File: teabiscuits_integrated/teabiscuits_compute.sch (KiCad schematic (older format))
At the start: 38 parts, among them J1 Barrel_Jack, J10 Conn_Coaxial, J2 Conn_02x04_Odd_Even, J3 Conn_01x03, J4 Conn_01x03, J5 Conn_02x03_Odd_Even, J6 J1B1211CCD, J7 Conn_Coaxial, J8 Conn_Coaxial, J9 Conn_01x03, U1 teensy41, U2 OP07, U3 OP07, U4 TLE2426xP, U5 LF398_SOIC8, U7 REF5025AD

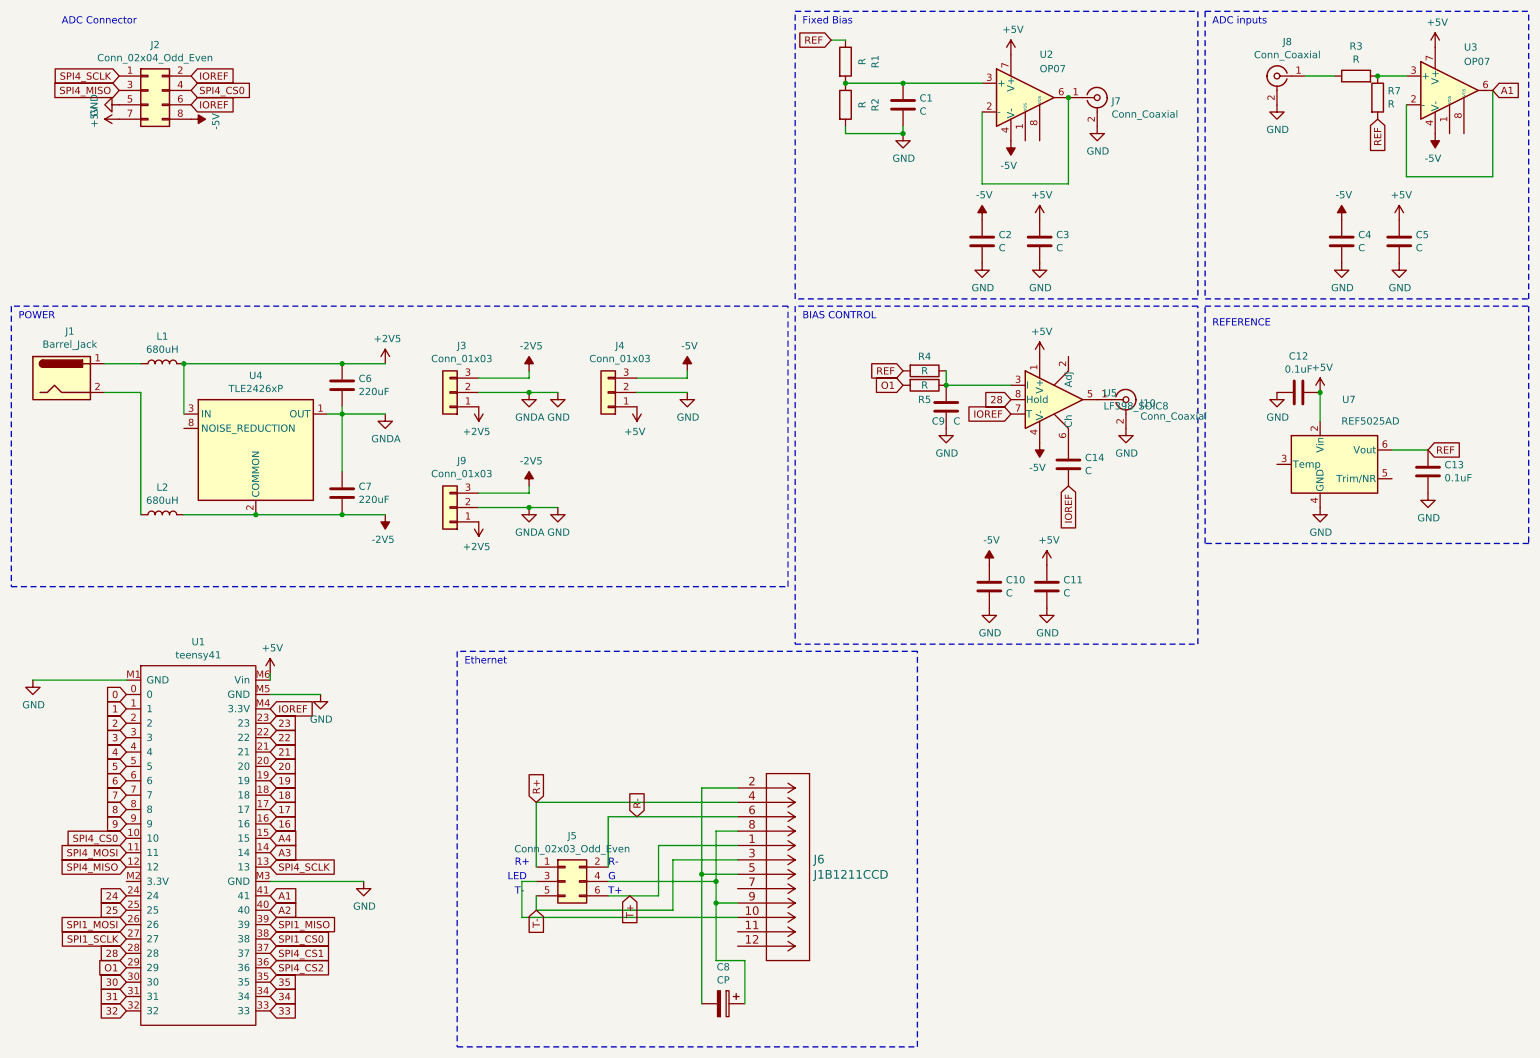
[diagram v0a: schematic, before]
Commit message: r4 of integrated pcb
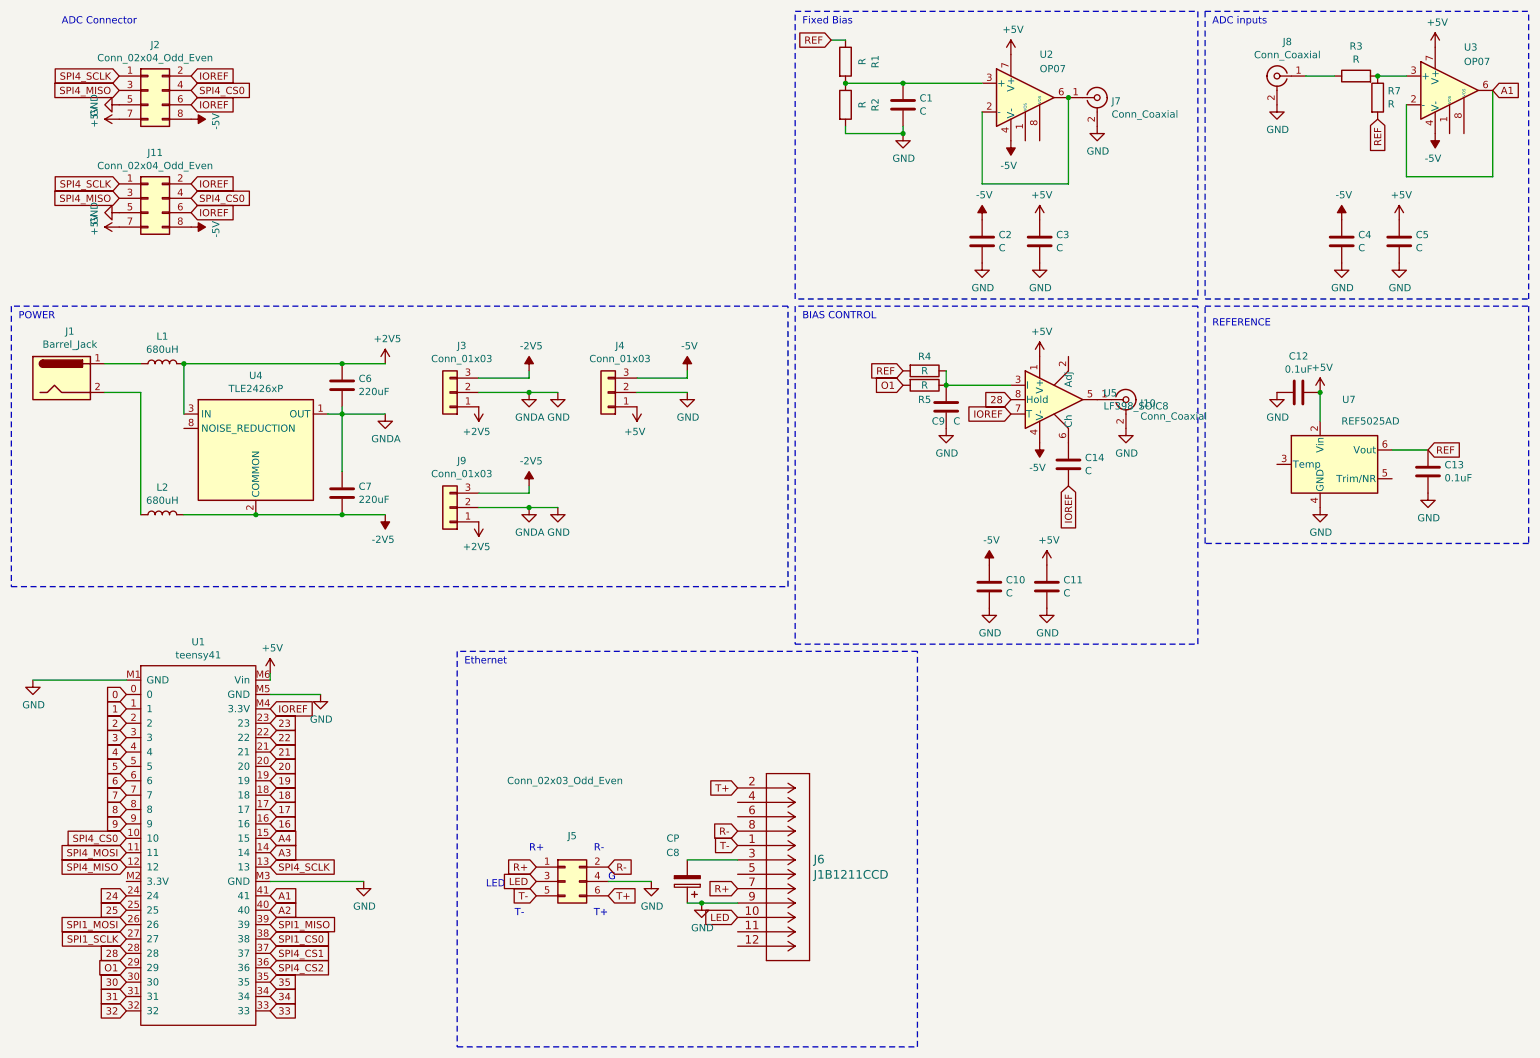
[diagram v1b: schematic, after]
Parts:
- added J11: Conn_02x04_Odd_Even, Connector_PinHeader_2.54mm:PinHeader_2x04_P2.54mm_Vertical, symbol Connector_Generic:Conn_02x04_Odd_Even
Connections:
- net +5V: now also J11.7 (Pin_7)
- net -5V: now also J11.8 (Pin_8)
- net GND: now also C8.1, J5.4 (Pin_4), J6.9, J11.5 (Pin_5)
- net IOREF: now also J11.2 (Pin_2), J11.6 (Pin_6)
- net R+: now also J6.7; no longer J6.4
- net R-: now also J6.8; no longer J6.6
- net SPI4_CS0: now also J11.4 (Pin_4)
- net SPI4_MISO: now also J11.3 (Pin_3)
- net SPI4_SCLK: now also J11.1 (Pin_1)
- net T+: now also J6.2; no longer J6.1
- net T-: now also J6.1; no longer J6.3
- net LED: now reaches J5.3 (Pin_3), J6.10
- new net: C8.2, J6.3
- now unconnected: J6.5
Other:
- moved on the sheet: C8
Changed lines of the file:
@@
 P 4450 6550
 F 0 "J5" H 4500 6867 50  0000 C CNN
-F 1 "Conn_02x03_Odd_Even" H 4500 6776 50  0000 C CNN
+F 1 "Conn_02x03_Odd_Even" H 4450 7250 50  0000 C CNN
 F 2 "Connector_PinHeader_2.00mm:PinHeader_2x03_P2.00mm_Vertical" H 4450 6550 50  0001 C CNN
 F 3 "~" H 4450 6550 50  0001 C CNN
@@
 L Device:CP C8
 U 1 1 5F594A00
-P 5550 7400
-F 0 "C8" V 5295 7400 50  0000 C CNN
-F 1 "CP" V 5386 7400 50  0000 C CNN
-F 2 "Capacitor_THT:C_Rect_L4.0mm_W2.5mm_P2.50mm" H 5588 7250 50  0001 C CNN
-F 3 "~" H 5550 7400 50  0001 C CNN
-	1    5550 7400
-	0    1    1    0
+P 5300 6550
+F 0 "C8" H 5400 6350 50  0000 C CNN
+F 1 "CP" H 5400 6250 50  0000 C CNN
+F 2 "Capacitor_THT:C_Rect_L4.0mm_W2.5mm_P2.50mm" H 5338 6400 50  0001 C CNN
+F 3 "~" H 5300 6550 50  0001 C CNN
+	1    5300 6550
+	-1   0    0    1
 $EndComp
 Wire Notes Line
@@
 	4400 3950 4200 3950
 Connection ~ 4200 3950
-Text Notes 4100 6450 0    50   ~ 0
+Text Notes 4200 6350 0    50   ~ 0
 R+
-Text Notes 4750 6450 0    50   ~ 0
+Text Notes 4650 6350 0    50   ~ 0
 R-
-Text Notes 4050 6550 0    50   ~ 0
+Text Notes 3900 6600 0    50   ~ 0
 LED
 Text Notes 4750 6550 0    50   ~ 0
 G
-Text Notes 4100 6650 0    50   ~ 0
+Text Notes 4100 6800 0    50   ~ 0
 T-
-Text Notes 4750 6650 0    50   ~ 0
+Text Notes 4650 6800 0    50   ~ 0
 T+
-Wire Wire Line
-	4750 6650 5100 6650
-Wire Wire Line
-	5100 6650 5100 6300
-Wire Wire Line
-	5100 6300 5650 6300
-Wire Wire Line
-	4250 6650 4250 6750
-Wire Wire Line
-	4250 6750 5200 6750
-Wire Wire Line
-	5200 6750 5200 6400
-Wire Wire Line
-	5200 6400 5650 6400
-Wire Wire Line
-	4250 6450 4250 6000
-Wire Wire Line
-	4250 6000 5650 6000
-Wire Wire Line
-	4750 6450 4750 6100
-Wire Wire Line
-	4750 6100 5650 6100
-Wire Wire Line
-	5650 6200 5500 6200
-Wire Wire Line
-	5500 6200 5500 6550
-Wire Wire Line
-	5500 6700 5650 6700
-Wire Wire Line
-	4750 6550 5500 6550
-Connection ~ 5500 6550
-Wire Wire Line
-	5500 6550 5500 6700
-Wire Wire Line
-	5650 6800 4150 6800
-Wire Wire Line
-	4150 6800 4150 6550
-Wire Wire Line
-	4150 6550 4250 6550
-Wire Wire Line
-	5650 5900 5400 5900
-Wire Wire Line
-	5400 5900 5400 6500
-Wire Wire Line
-	5400 6500 5650 6500
-Wire Wire Line
-	5400 6500 5400 7400
-Connection ~ 5400 6500
-Wire Wire Line
-	5700 7400 5700 7100
-Wire Wire Line
-	5700 7100 5500 7100
-Wire Wire Line
-	5500 7100 5500 6700
-Connection ~ 5500 6700
-Text GLabel 4250 6750 3    50   Input ~ 0
+Text GLabel 4250 6650 0    50   Input ~ 0
 T-
-Text GLabel 4900 6650 3    50   Input ~ 0
+Text GLabel 4750 6650 2    50   Input ~ 0
 T+
-Text GLabel 4950 6100 1    50   Input ~ 0
+Text GLabel 5650 6200 0    50   Input ~ 0
 R-
-Text GLabel 4250 6000 1    50   Input ~ 0
+Text GLabel 5650 6600 0    50   Input ~ 0
 R+
 $Comp
@@
 	1    0    0    -1
 $EndComp
+$Comp
+L Connector_Generic:Conn_02x04_Odd_Even J11
+U 1 1 5F77C0F4
+P 1550 1800
+F 0 "J11" H 1600 2117 50  0000 C CNN
+F 1 "Conn_02x04_Odd_Even" H 1600 2026 50  0000 C CNN
+F 2 "Connector_PinHeader_2.54mm:PinHeader_2x04_P2.54mm_Vertical" H 1550 1800 50  0001 C CNN
+F 3 "~" H 1550 1800 50  0001 C CNN
+	1    1550 1800
+	1    0    0    -1
+$EndComp
+Text GLabel 1350 1700 0    50   Input ~ 0
+SPI4_SCLK
+Text GLabel 1850 1700 2    50   Input ~ 0
+IOREF
+Text GLabel 1850 1900 2    50   Input ~ 0
+IOREF
+Text GLabel 1850 1800 2    50   Input ~ 0
+SPI4_CS0
+Text GLabel 1350 1800 0    50   Input ~ 0
+SPI4_MISO
+$Comp
+L power:+5V #PWR0123
+U 1 1 5F77C103
+P 1350 2000
+F 0 "#PWR0123" H 1350 1850 50  0001 C CNN
+F 1 "+5V" H 1365 2173 50  0000 C CNN
+F 2 "" H 1350 2000 50  0001 C CNN
+F 3 "" H 1350 2000 50  0001 C CNN
+	1    1350 2000
+	0    -1   -1   0
+$EndComp
+$Comp
+L power:GND #PWR0124
+U 1 1 5F77C10D
+P 1350 1900
+F 0 "#PWR0124" H 1350 1650 50  0001 C CNN
+F 1 "GND" H 1355 1727 50  0000 C CNN
+F 2 "" H 1350 1900 50  0001 C CNN
+F 3 "" H 1350 1900 50  0001 C CNN
+	1    1350 1900
+	0    1    1    0
+$EndComp
+$Comp
+L power:-5V #PWR0125
+U 1 1 5F77C117
+P 1850 2000
+F 0 "#PWR0125" H 1850 2100 50  0001 C CNN
+F 1 "-5V" H 1865 2173 50  0000 C CNN
+F 2 "" H 1850 2000 50  0001 C CNN
+F 3 "" H 1850 2000 50  0001 C CNN
+	1    1850 2000
+	0    1    1    0
+$EndComp
+Text GLabel 5650 5900 0    50   Input ~ 0
+T+
+Text GLabel 4750 6450 2    50   Input ~ 0
+R-
+Text GLabel 5650 6300 0    50   Input ~ 0
+T-
+Text GLabel 4250 6450 0    50   Input ~ 0
+R+
+Text GLabel 4250 6550 0    50   Input ~ 0
+LED
+Text GLabel 5650 6800 0    50   Input ~ 0
+LED
+$Comp
+L power:GND #PWR0126
+U 1 1 5F6EEB3C
+P 5050 6550
+F 0 "#PWR0126" H 5050 6300 50  0001 C CNN
+F 1 "GND" H 5055 6377 50  0000 C CNN
+F 2 "" H 5050 6550 50  0001 C CNN
+F 3 "" H 5050 6550 50  0001 C CNN
+	1    5050 6550
+	1    0    0    -1
+$EndComp
+$Comp
+L power:GND #PWR0127
+U 1 1 5F6EED08
+P 5400 6700
+F 0 "#PWR0127" H 5400 6450 50  0001 C CNN
+F 1 "GND" H 5405 6527 50  0000 C CNN
+F 2 "" H 5400 6700 50  0001 C CNN
+F 3 "" H 5400 6700 50  0001 C CNN
+	1    5400 6700
+	1    0    0    -1
+$EndComp
+Wire Wire Line
+	5650 6700 5400 6700
+Wire Wire Line
+	5050 6550 4750 6550
+Wire Wire Line
+	5650 6400 5300 6400
+Wire Wire Line
+	5300 6700 5400 6700
+Connection ~ 5400 6700
 $EndSCHEMATC
